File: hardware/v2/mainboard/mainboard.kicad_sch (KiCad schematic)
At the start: 19 parts, among them J1 LEG1_RJ11, J2 LEG2_RJ11, J3 LEG3_RJ11, J4 LEG4_RJ11, J5 LEG5_RJ11, J6 LEG6_RJ11, J7 SBEC_5V_IN, J8 3V3_REG_MODULE, J9 IMU_I2C, U1 ESP32-WROOM-32D, U2 SP3485CN

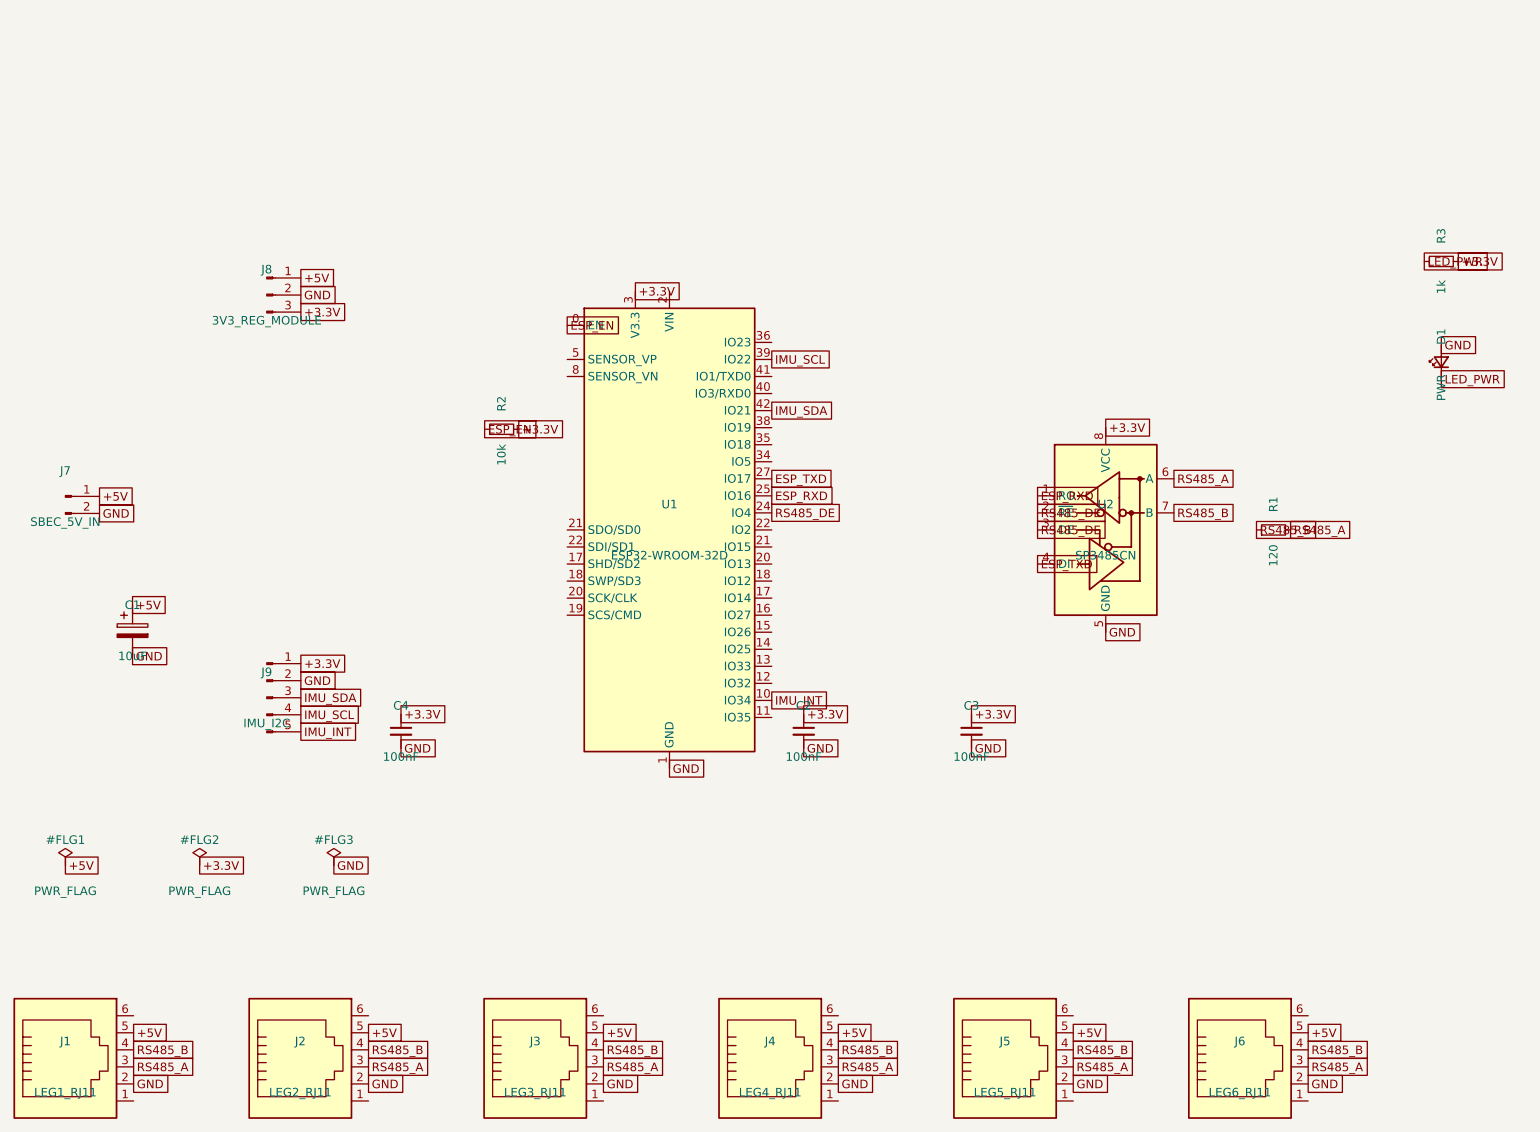
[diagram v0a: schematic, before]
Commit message: manual fixes for mainboard
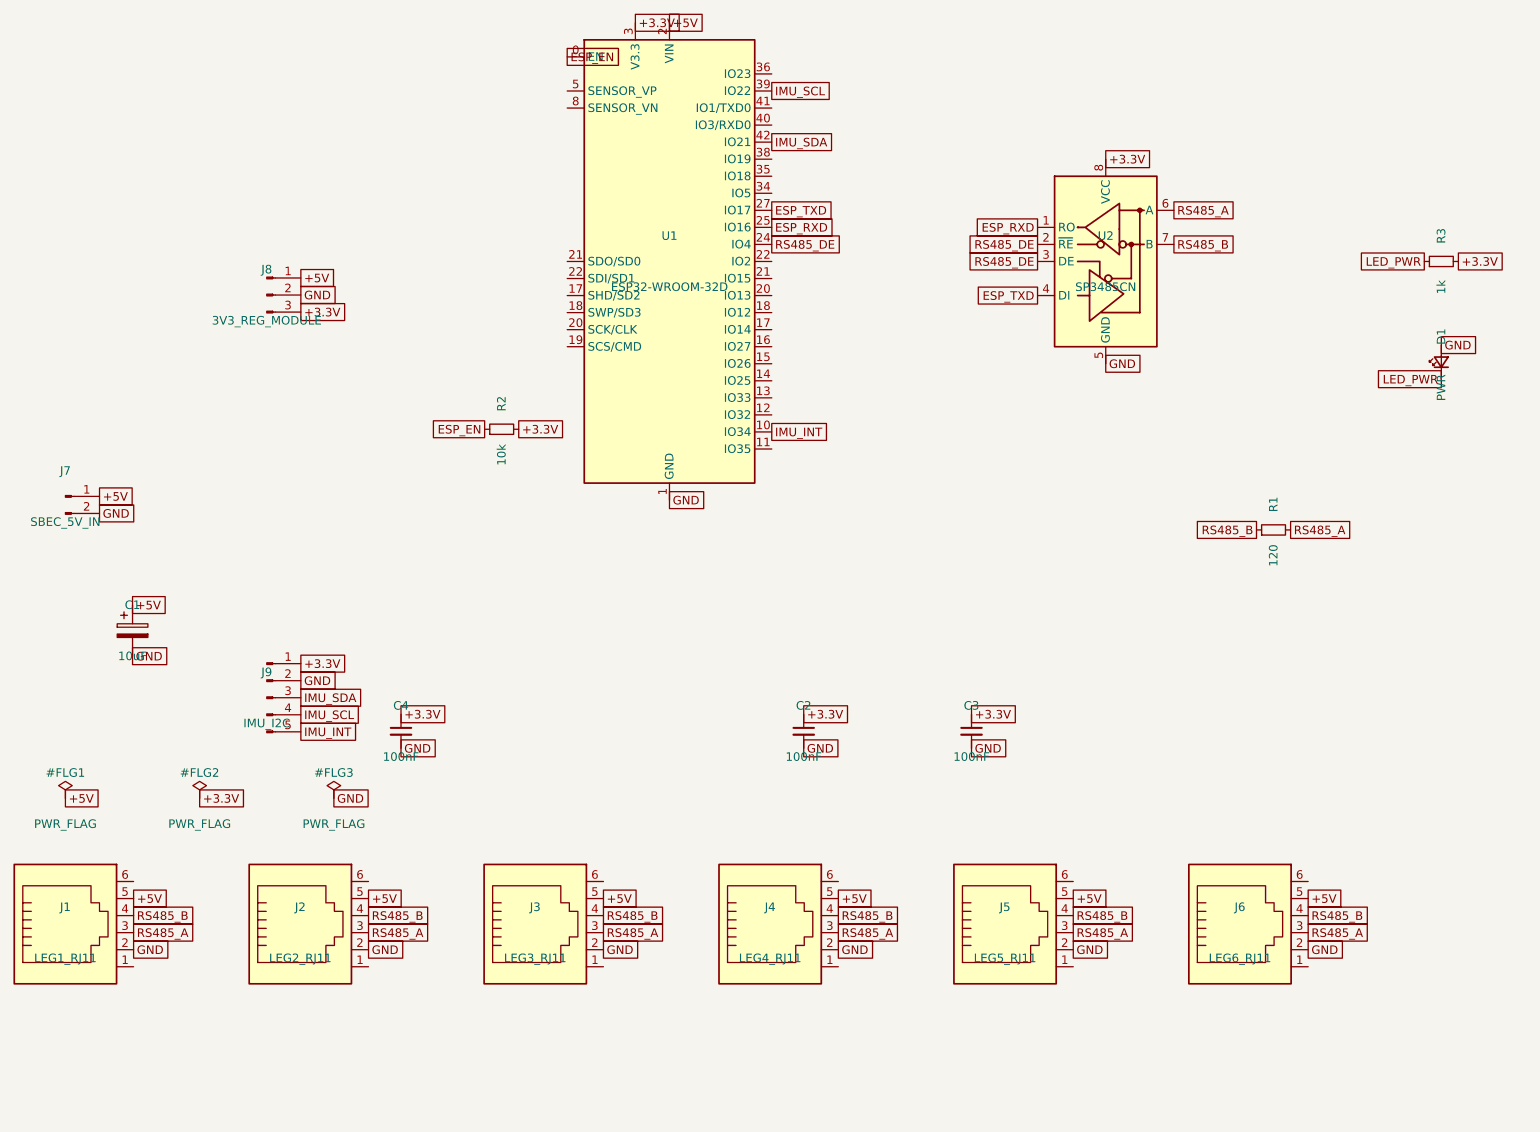
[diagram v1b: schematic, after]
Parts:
- C1: footprint Capacitor_SMD:C_0805_2012Metric -> Capacitor_THT:CP_Radial_D4.0mm_P2.00mm
- J7: footprint (none) -> TerminalBlock:TerminalBlock_MaiXu_MX126-5.0-02P_1x02_P5.00mm
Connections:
- net +5V: now also U1.2 (VIN)
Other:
- moved on the sheet: J1, J2, J3, J4, J5, J6, U1, U2
